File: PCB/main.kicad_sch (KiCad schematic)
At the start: 19 parts, among them SW1 Switch, SW2 Switch, SW3 Switch, SW4 Switch, SW5 Switch, SW6 Switch, SW7 Switch, SW8 Switch, SW9 Switch

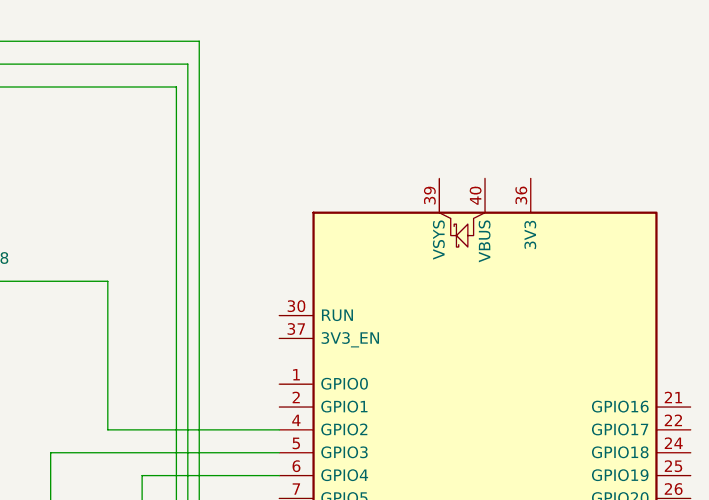
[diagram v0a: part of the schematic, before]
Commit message: fixed problem wirh scamatic
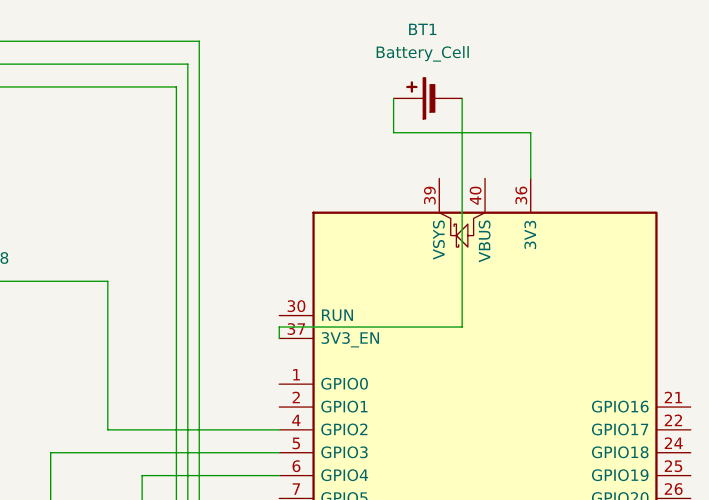
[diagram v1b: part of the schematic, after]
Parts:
- added BT1: Battery_Cell, symbol Device:Battery_Cell
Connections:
- net at A1.36 (3V3): now also BT1.1 (+)
- net at A1.37 (3V3_EN): now also BT1.2 (-)
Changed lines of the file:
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@@
+	(wire
+		(pts
+			(xy 210.82 55.88) (xy 210.82 57.15)
+		)
+		(stroke
+			(width 0)
+			(type default)
+		)
+	)
 	(wire
 		(pts
@@
 	(wire
 		(pts
+			(xy 238.76 34.29) (xy 238.76 39.37)
+		)
+		(stroke
+			(width 0)
+			(type default)
+		)
+	)
+	(wire
+		(pts
 			(xy 129.54 43.18) (xy 129.54 78.74)
 		)
@@
 	(wire
 		(pts
+			(xy 231.14 55.88) (xy 210.82 55.88)
+		)
+		(stroke
+			(width 0)
+			(type default)
+		)
+	)
+	(wire
+		(pts
+			(xy 231.14 30.48) (xy 231.14 55.88)
+		)
+		(stroke
+			(width 0)
+			(type default)
+		)
+	)
+	(wire
+		(pts
 			(xy 139.7 86.36) (xy 171.45 86.36)
 		)
@@
 	(wire
 		(pts
+			(xy 223.52 30.48) (xy 223.52 34.29)
+		)
+		(stroke
+			(width 0)
+			(type default)
+		)
+	)
+	(wire
+		(pts
 			(xy 129.54 26.67) (xy 129.54 43.18)
 		)
@@
 		(pts
 			(xy 104.14 86.36) (xy 139.7 86.36)
+		)
+		(stroke
+			(width 0)
+			(type default)
+		)
+	)
+	(wire
+		(pts
+			(xy 223.52 34.29) (xy 238.76 34.29)
 		)
 		(stroke
@@
 					(unit 1)
 				)
+			)
+		)
+	)
+	(symbol
+		(lib_id "Device:Battery_Cell")
+		(at 228.6 30.48 90)
+		(unit 1)
+		(exclude_from_sim no)
+		(in_bom yes)
+		(on_board yes)
+		(dnp no)
+		(fields_autoplaced yes)
+		(property "Reference" "BT1"
+			(at 226.7585 22.86 90)
+			(effects
+				(font
+					(size 1.27 1.27)
+				)
+			)
+		)
+		(property "Value" "Battery_Cell"
+			(at 226.7585 25.4 90)
+			(effects
+				(font
+					(size 1.27 1.27)
+				)
+			)
+		)
+		(property "Footprint" ""
+			(at 227.076 30.48 90)
+			(effects
+				(font
+					(size 1.27 1.27)
+				)
+				(hide yes)
+			)
+		)
+		(property "Datasheet" "~"
+			(at 227.076 30.48 90)
+			(effects
+				(font
+					(size 1.27 1.27)
+				)
+				(hide yes)
+			)
+		)
+		(property "Description" "Single-cell battery"
+			(at 228.6 30.48 0)
+			(effects
+				(font
+					(size 1.27 1.27)
+				)
+				(hide yes)
+			)
+		)
+		(pin "1"
+		)
+		(pin "2"
+		)
+		(instances
+			(project ""
+				(path "/b69ac572-6c4c-4447-98a7-d329fd5fffbd"
+					(reference "BT1")
+					(unit 1)
+				)
